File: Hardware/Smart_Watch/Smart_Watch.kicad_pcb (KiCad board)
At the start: 2 copper layers, 40 x 40 mm, 57 parts, among them J1 USB_C_Receptacle_USB2.0, SW1 PICO BOOT, SW2 PICO RST, U1 W25Q128JVS, U2 RP2040, U3 TLV62568DBV, U4 TLV62568DBV, Y1 12.000MHZ

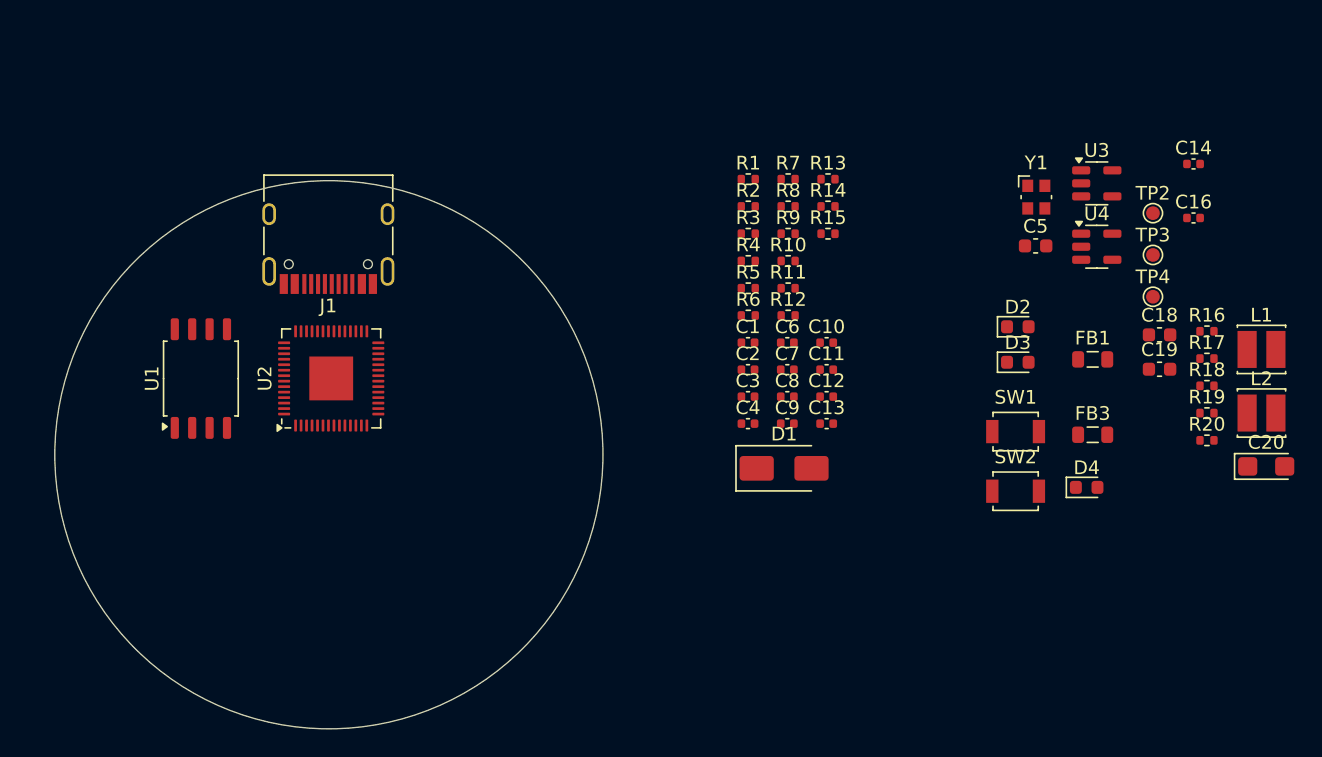
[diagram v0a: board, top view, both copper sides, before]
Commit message: update layout pcb
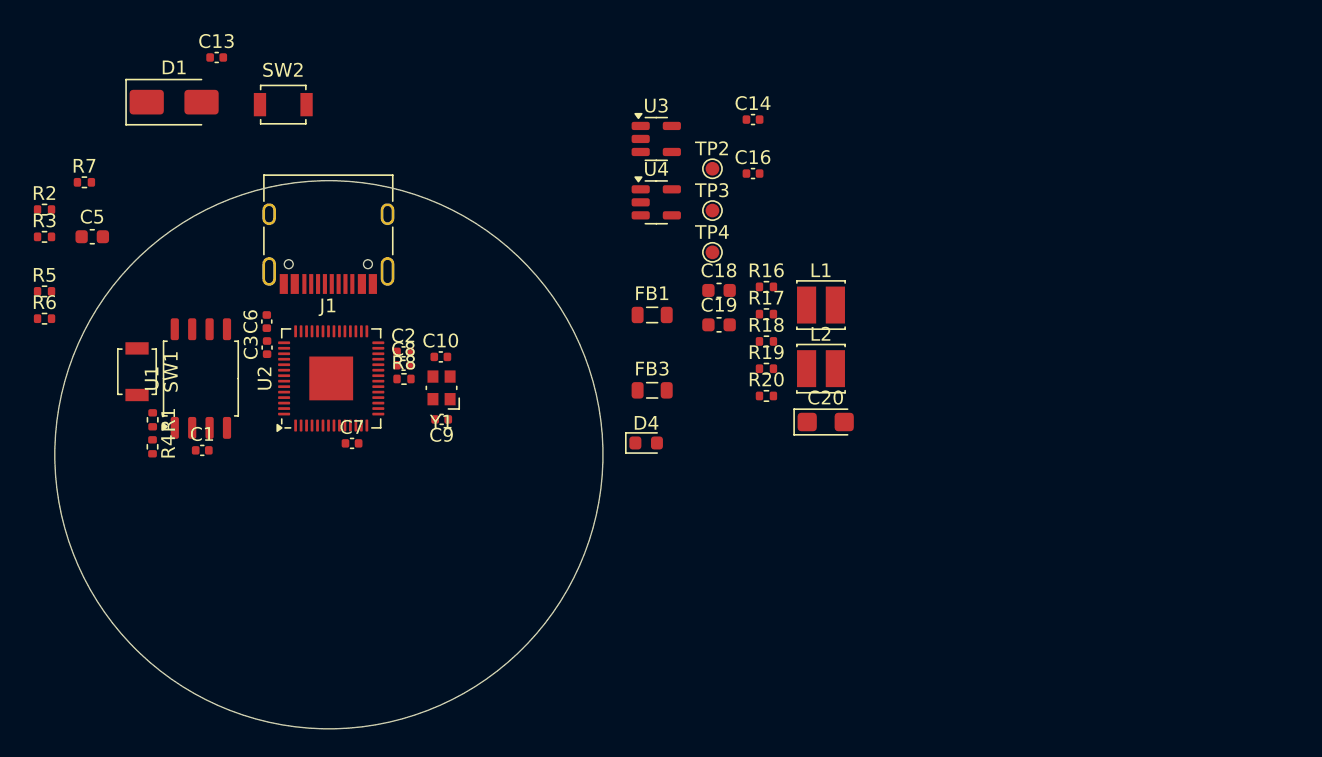
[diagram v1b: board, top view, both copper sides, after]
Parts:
- removed C11, C12, C4: 100nF, Capacitor_SMD:C_0402_1005Metric
- removed D2, D3: LED, LED_SMD:LED_0603_1608Metric
- removed R10, R11, R12, R13, R9: 22R, Resistor_SMD:R_0402_1005Metric
- removed R14, R15: 330R, Resistor_SMD:R_0402_1005Metric
- moved C5 68.8 mm to (108.6, 39.7)
- moved SW1 64.3 mm to (111.8, 49.5), turned to -90 degrees
- moved SW2 60.4 mm to (122.5, 30.0)
- moved C13 51.9 mm to (117.7, 26.6)
- moved D1 51.9 mm to (114.6, 29.9)
- moved R7 51.4 mm to (108.0, 35.7)
- moved R2 51.4 mm to (105.1, 37.7)
- moved R3 51.4 mm to (105.1, 39.7)
- moved R5 51.4 mm to (105.1, 43.7)
- moved R6 51.4 mm to (105.1, 45.7)
- moved R1 46.9 mm to (113.0, 53.0), turned to -90 degrees
- moved Y1 45.6 mm to (134.1, 50.7), turned to 180 degrees
- moved R4 45.5 mm to (113.0, 55.0), turned to -90 degrees
- moved C1 40.6 mm to (116.6, 55.3)
- moved C6 38.0 mm to (121.3, 45.9), turned to 90 degrees
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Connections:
- U2 pad 11: FPGA_MISO -> unconnected-(U2-GPIO8-Pad11)
- U2 pad 12: FPGA_SDCS -> unconnected-(U2-GPIO9-Pad12)
- U2 pad 13: Net-(U2-GPIO10) -> unconnected-(U2-GPIO10-Pad13)
- U2 pad 14: FPGA_MOSI -> unconnected-(U2-GPIO11-Pad14)
- U2 pad 15: /RP2040/TXD -> unconnected-(U2-GPIO12-Pad15)
- U2 pad 16: /RP2040/RXD -> unconnected-(U2-GPIO13-Pad16)
- U2 pad 17: Net-(U2-GPIO14) -> unconnected-(U2-GPIO14-Pad17)
- U2 pad 18: Net-(U2-GPIO15) -> unconnected-(U2-GPIO15-Pad18)
- U2 pad 2: /RP2040/GP0 -> unconnected-(U2-GPIO0-Pad2)
- U2 pad 27: TDI -> unconnected-(U2-GPIO16-Pad27)
- U2 pad 28: TDO -> unconnected-(U2-GPIO17-Pad28)
- U2 pad 29: TCK -> unconnected-(U2-GPIO18-Pad29)
- U2 pad 3: /RP2040/GP1 -> unconnected-(U2-GPIO1-Pad3)
- U2 pad 30: TMS -> unconnected-(U2-GPIO19-Pad30)
- U2 pad 31: /RP2040/GP20 -> unconnected-(U2-GPIO20-Pad31)
- U2 pad 32: /RP2040/GP21 -> unconnected-(U2-GPIO21-Pad32)
- U2 pad 34: /RP2040/GP22 -> unconnected-(U2-GPIO22-Pad34)
- U2 pad 35: /RP2040/GP23 -> unconnected-(U2-GPIO23-Pad35)
- U2 pad 36: Net-(U2-GPIO24) -> unconnected-(U2-GPIO24-Pad36)
- U2 pad 37: Net-(U2-GPIO25) -> unconnected-(U2-GPIO25-Pad37)
- U2 pad 38: Net-(U2-GPIO26_ADC0) -> unconnected-(U2-GPIO26_ADC0-Pad38)
- U2 pad 39: Net-(U2-GPIO27_ADC1) -> unconnected-(U2-GPIO27_ADC1-Pad39)
- U2 pad 4: /RP2040/GP2 -> unconnected-(U2-GPIO2-Pad4)
- U2 pad 5: /RP2040/GP3 -> unconnected-(U2-GPIO3-Pad5)
- U2 pad 6: /RP2040/GP4 -> unconnected-(U2-GPIO4-Pad6)
- U2 pad 7: /RP2040/GP5 -> unconnected-(U2-GPIO5-Pad7)
- U2 pad 8: /RP2040/GP6 -> unconnected-(U2-GPIO6-Pad8)
- U2 pad 9: /RP2040/GP7 -> unconnected-(U2-GPIO7-Pad9)
